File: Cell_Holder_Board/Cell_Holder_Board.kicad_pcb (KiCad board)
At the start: 2 copper layers, 126.5 x 76.1 mm, 24 parts, among them J1 ntc 10k, SW1 BMS_RESET, U1 MP2615

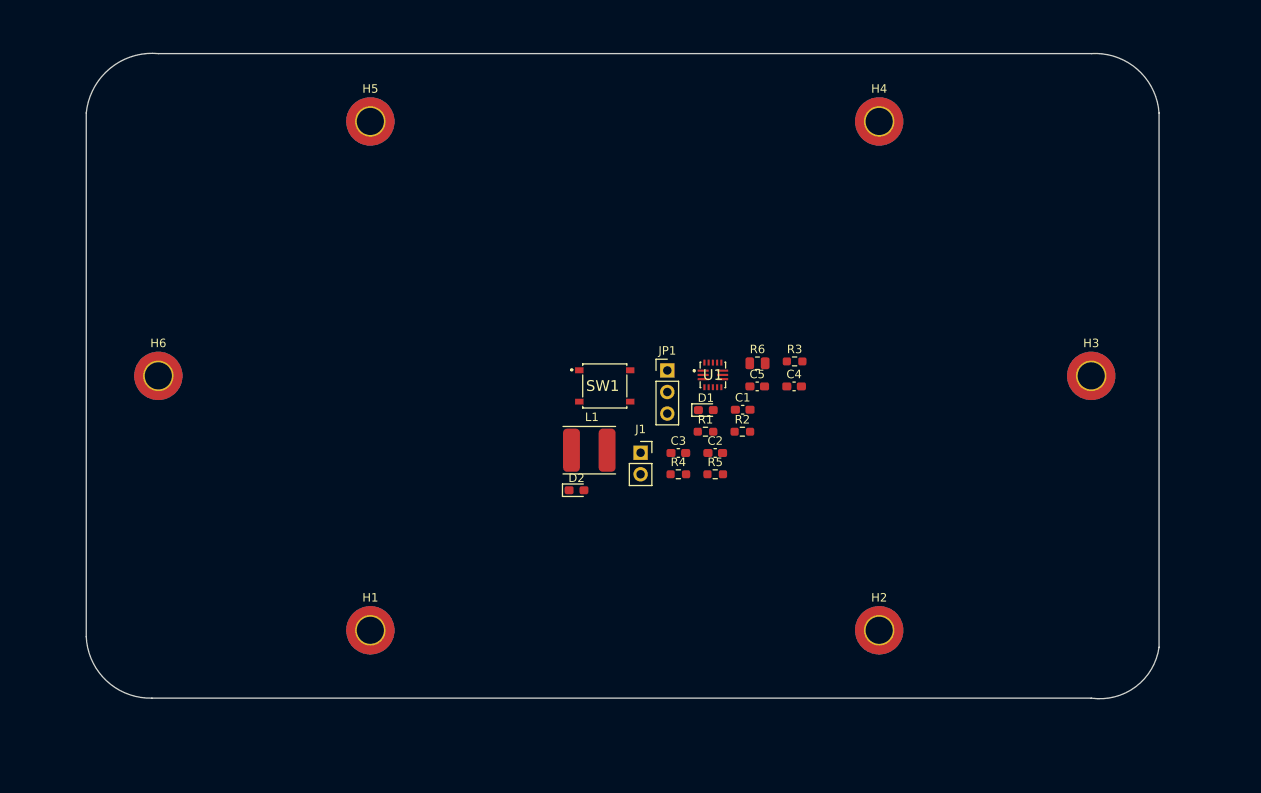
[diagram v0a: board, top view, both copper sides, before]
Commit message: v
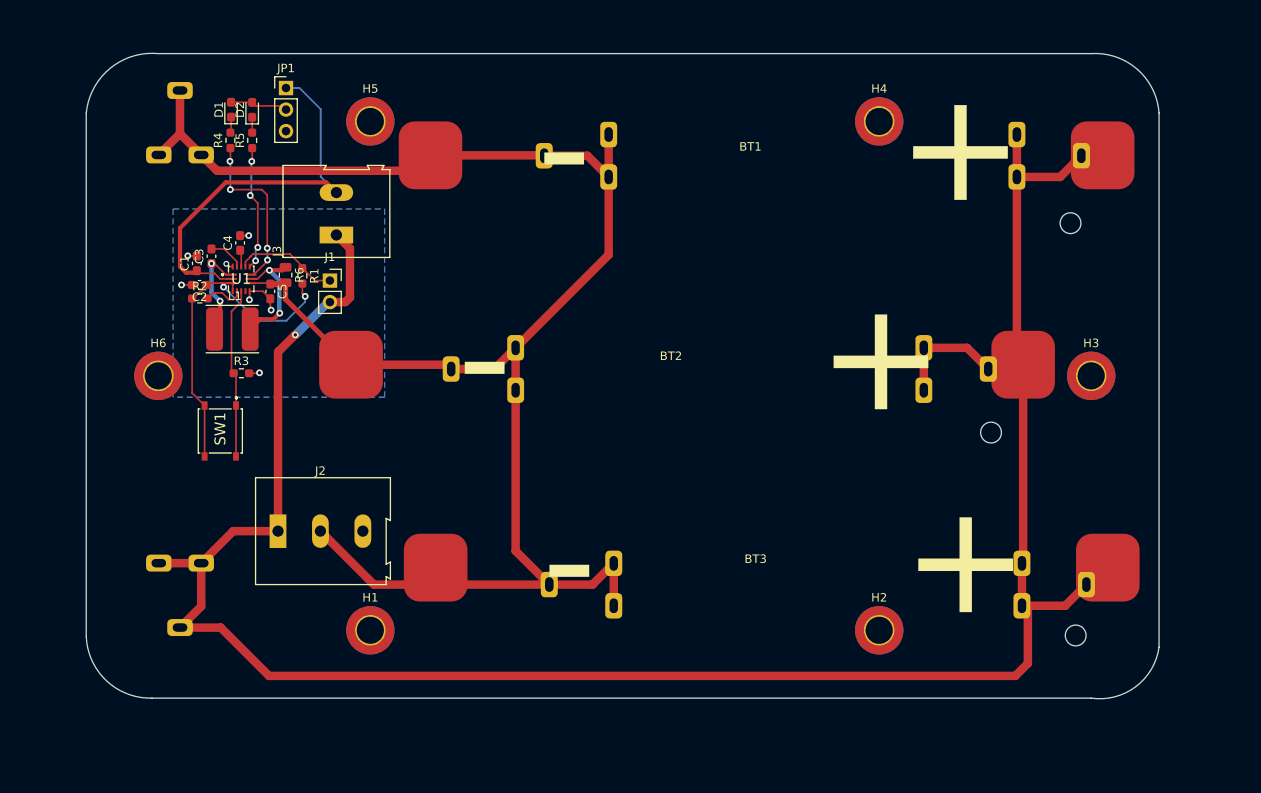
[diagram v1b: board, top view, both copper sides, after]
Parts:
- added BT1: 18650_SMD_top, Z_mycustom_footprint_lib:MYOUNG BH 18650 B1BA002, F.Cu at (159.0, 46.9)
- added BT2: 18650_SMD_top, Z_mycustom_footprint_lib:MYOUNG BH 18650 B1BA002, F.Cu at (149.6, 71.6)
- added BT3: 18650_SMD_top, Z_mycustom_footprint_lib:MYOUNG BH 18650 B1BA002, F.Cu at (159.6, 95.5)
- added BT5: 18650_THT_bottom, Z_mycustom_footprint_lib:MYOUNG MY-18650-01, B.Cu at (52.7, 46.9)
- added BT6: 18650_THT_bottom, Z_mycustom_footprint_lib:MYOUNG MY-18650-01, B.Cu at (101.4, 95.0)
- added BT7: 18650_THT_bottom, Z_mycustom_footprint_lib:MYOUNG MY-18650-01, B.Cu at (100.8, 44.5)
- added BT8: 18650_THT_bottom, Z_mycustom_footprint_lib:MYOUNG MY-18650-01, B.Cu at (89.8, 69.6)
- added J2: IN/OUT, TerminalBlock:TerminalBlock_Altech_AK300-3_P5.00mm, F.Cu at (61.8, 91.2)
- added J3: IN/OUT, TerminalBlock:TerminalBlock_Altech_AK300-2_P5.00mm, F.Cu at (68.7, 56.3)
- moved C4 67.5 mm to (57.3, 57.3), turned to 90 degrees
- moved R5 67.3 mm to (58.7, 45.2), turned to 90 degrees
- moved C1 66.6 mm to (52.2, 59.7), turned to 90 degrees
- moved D1 66.2 mm to (56.2, 41.5), turned to 90 degrees
- moved R4 65.9 mm to (56.2, 45.2), turned to 90 degrees
- moved R2 65.9 mm to (52.6, 63.8)
- moved R3 65.2 mm to (57.5, 72.6)
- moved C2 63.9 mm to (52.5, 62.2), turned to 180 degrees
- moved C3 59.7 mm to (53.9, 58.8), turned to 90 degrees
- moved D2 58.9 mm to (58.7, 41.6), turned to 90 degrees
- moved C5 58.5 mm to (60.9, 63.0), turned to -90 degrees
- moved U1 56.8 mm to (57.4, 61.5)
- moved R6 56.6 mm to (62.7, 61.0), turned to -90 degrees
- moved JP1 56.0 mm to (62.7, 39.0)
- moved R1 51.0 mm to (64.6, 61.1), turned to -90 degrees
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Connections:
- H1 pad 1: GND -> unconnected-(H1-Pad1)
- H2 pad 1: GND -> unconnected-(H2-Pad1)
- H3 pad 1: GND -> unconnected-(H3-Pad1)
- H4 pad 1: GND -> unconnected-(H4-Pad1)
- H5 pad 1: GND -> unconnected-(H5-Pad1)
- H6 pad 1: GND -> unconnected-(H6-Pad1)
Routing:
- net GND: track 0.00 -> 276.5 mm, vias 0 -> 8
- net +BATT: track 0.00 -> 206.5 mm, vias 0 -> 1
- net Net-(C1-Pad1): track 0.00 -> 48.3 mm
- net /VCC: track 0.00 -> 40.6 mm, vias 0 -> 2
- net /~{EN}: track 0.00 -> 20.2 mm
- net Net-(R4-Pad1): track 0.00 -> 19.9 mm, vias 0 -> 4
- net /CSP: track 0.00 -> 16.5 mm, vias 0 -> 2
- net Net-(R5-Pad1): track 0.00 -> 14.8 mm, vias 0 -> 4
- net /NTC: track 0.00 -> 12.3 mm
- net /SW: track 0.00 -> 11.3 mm, vias 0 -> 2
- net /BMS_LED: track 0.00 -> 6.83 mm
- net /SEL: track 0.00 -> 4.84 mm
- net /BST: track 0.00 -> 4.20 mm
- net /TMR: track 0.00 -> 1.98 mm
- net Net-(D1-Pad1): track 0.00 -> 1.86 mm
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- added copper zone on B.Cu, net GND

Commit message: f
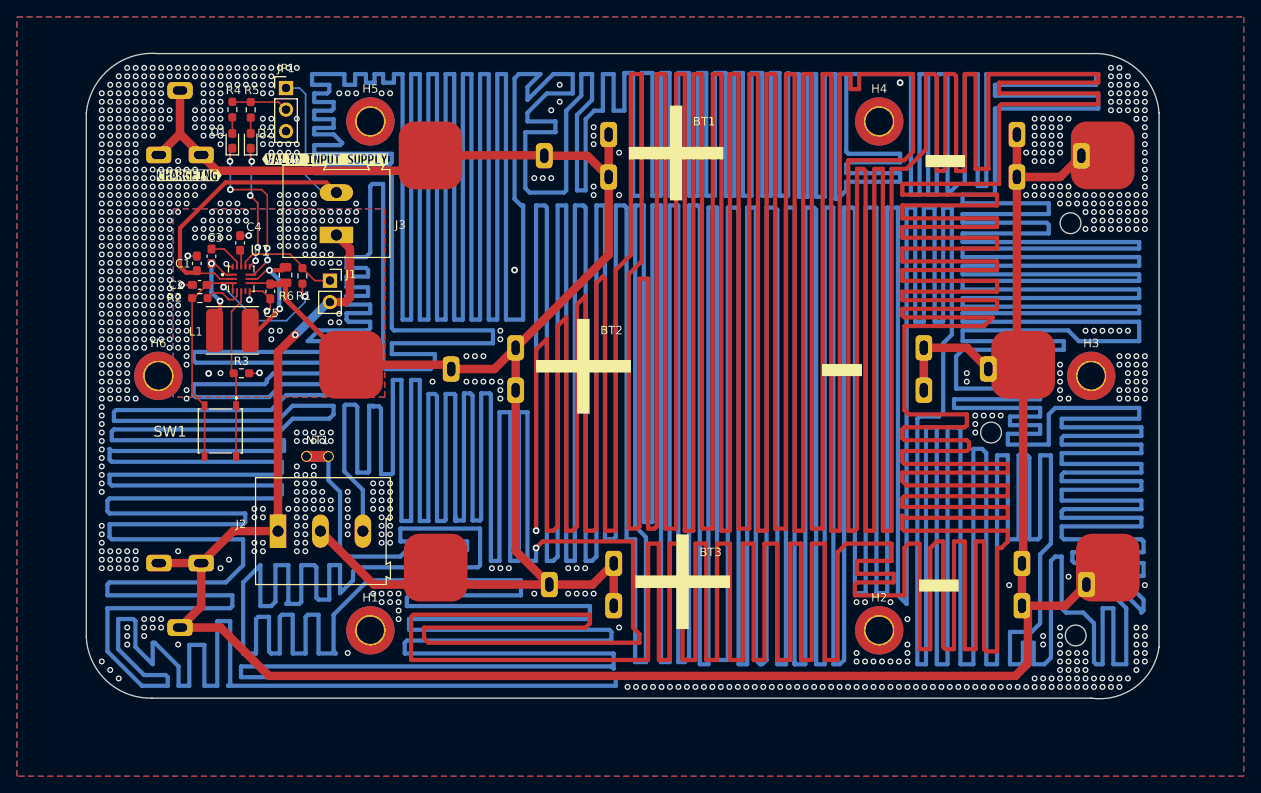
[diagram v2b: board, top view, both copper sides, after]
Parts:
- added NT1: NetTie_2, NetTie:NetTie-2_THT_Pad1.0mm, F.Cu at (65.1, 82.4)
- added kibuzzard-63738E7A: G***, kibuzzard-63738E7A, F.Cu at (67.3, 47.4)
- added kibuzzard-63738EBD: G***, kibuzzard-63738EBD, F.Cu at (51.3, 49.3)
- moved D1 3.67 mm to (56.4, 45.2)
- moved D2 3.66 mm to (58.5, 45.2)
- moved R4 3.64 mm to (56.4, 41.5)
- moved R5 3.61 mm to (58.5, 41.6)
- moved L1 0.15 mm to (54.3, 67.6)
- moved R2 0.05 mm to (52.6, 63.8)
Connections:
- D1 pad 1: Net-(D1-Pad1) -> Net-(U1-Pad11)
- D1 pad 2: /BMS_LED -> Net-(R4-Pad1)
- D2 pad 1: Net-(D2-Pad1) -> Net-(U1-Pad12)
- D2 pad 2: /BMS_LED -> Net-(R5-Pad1)
- R4 pad 2: Net-(D1-Pad1) -> /BMS_LED
- R5 pad 2: Net-(D2-Pad1) -> /BMS_LED
- U1 pad 11: Net-(R4-Pad1) -> Net-(U1-Pad11)
- U1 pad 12: Net-(R5-Pad1) -> Net-(U1-Pad12)
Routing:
- net /Heater: track 0.00 -> 8407.7 mm, vias 0 -> 2
- net Net-(U1-Pad11): track 0.00 -> 20.0 mm, vias 0 -> 4
- net Net-(R4-Pad1): track 19.9 -> 2.00 mm, vias 4 -> 0
- net Net-(U1-Pad12): track 0.00 -> 14.9 mm, vias 0 -> 4
- net Net-(R5-Pad1): track 14.8 -> 1.87 mm, vias 4 -> 0
- net +BATT: track 206.5 -> 204.1 mm
- net Net-(D1-Pad1): track 1.86 -> 0.00 mm
- net Net-(D2-Pad1): track 1.82 -> 0.00 mm
- net Net-(C1-Pad1): track 48.3 -> 49.2 mm
- net GND: track 276.5 -> 276.7 mm, vias 8 -> 962
- added copper zone on F.Cu, net GND
